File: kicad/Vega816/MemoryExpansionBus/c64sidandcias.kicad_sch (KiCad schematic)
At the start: 7 parts, among them J62 IRQ_OUT, J63 Device Select, J64 A/D Bus, J72 $80 (32B), J76 $00 (16B), J77 $40 (16B)

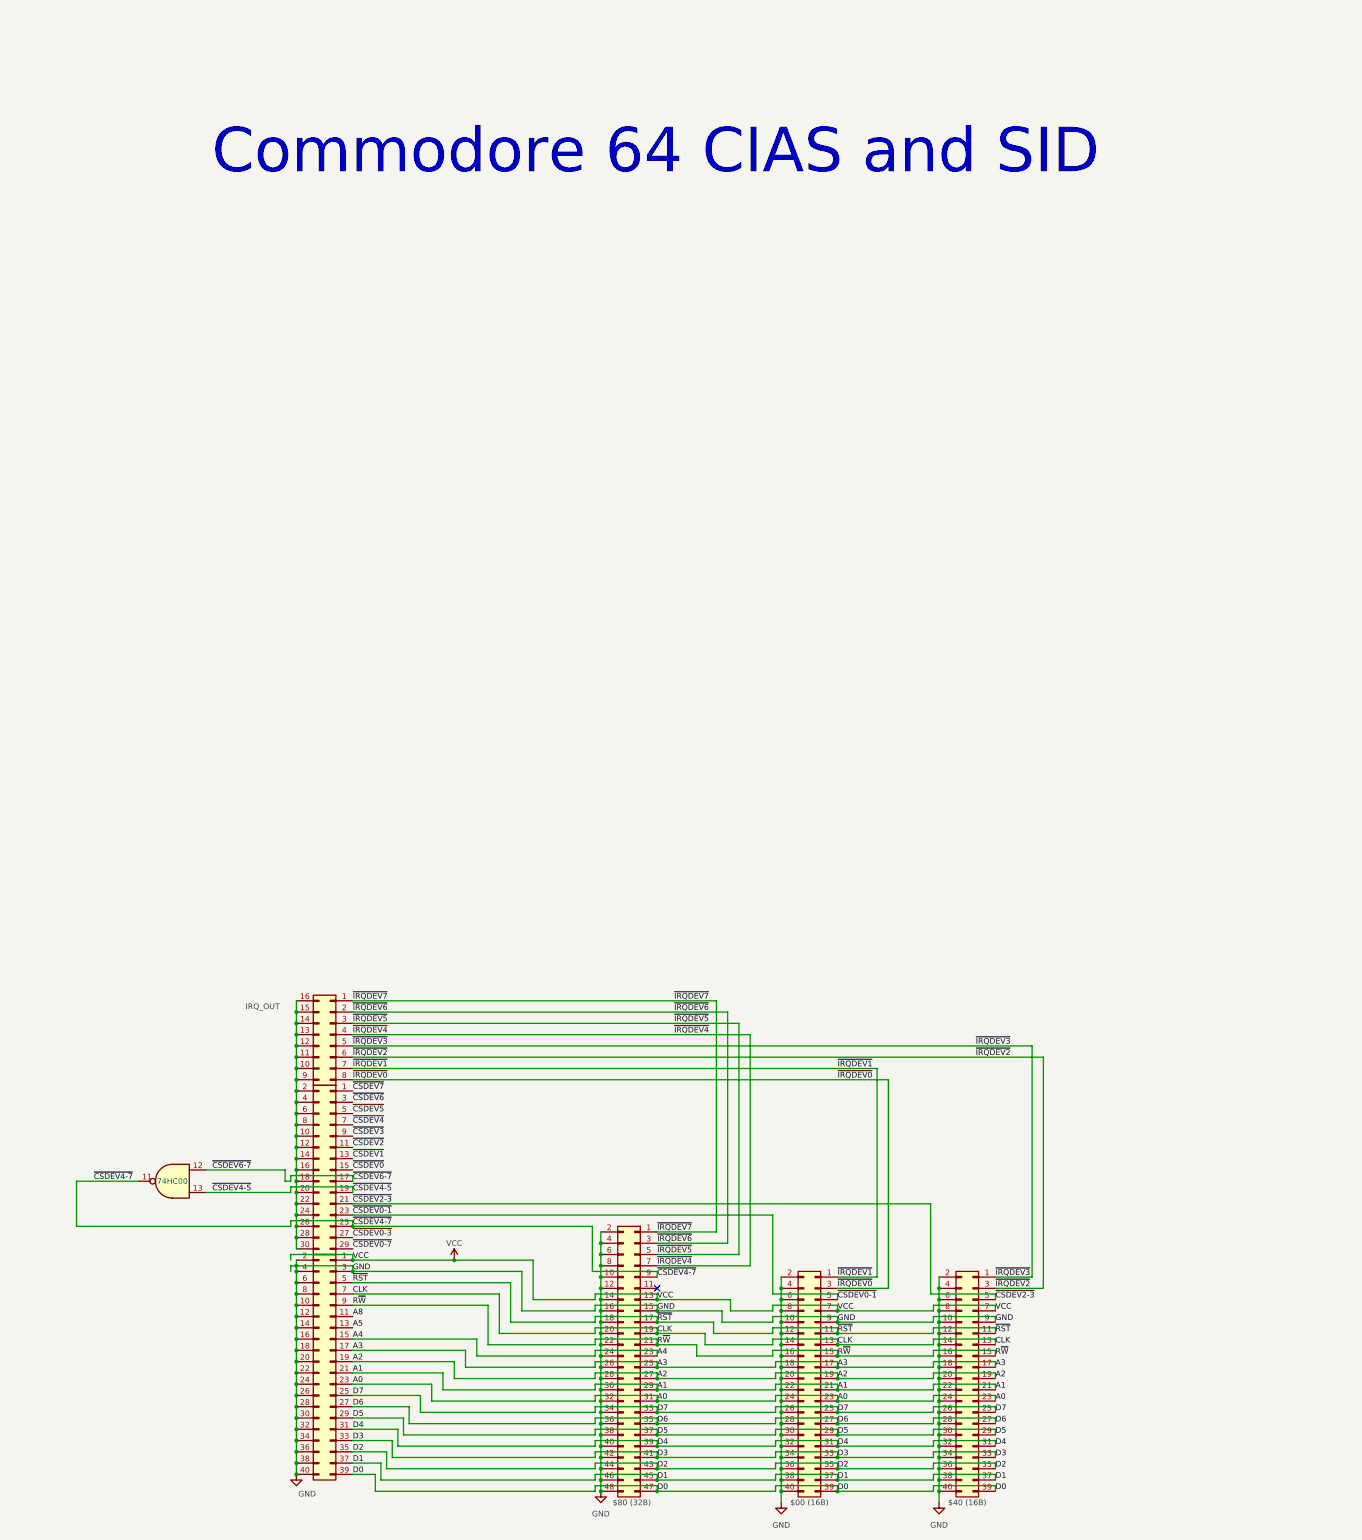
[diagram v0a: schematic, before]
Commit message: expansion port hi ram
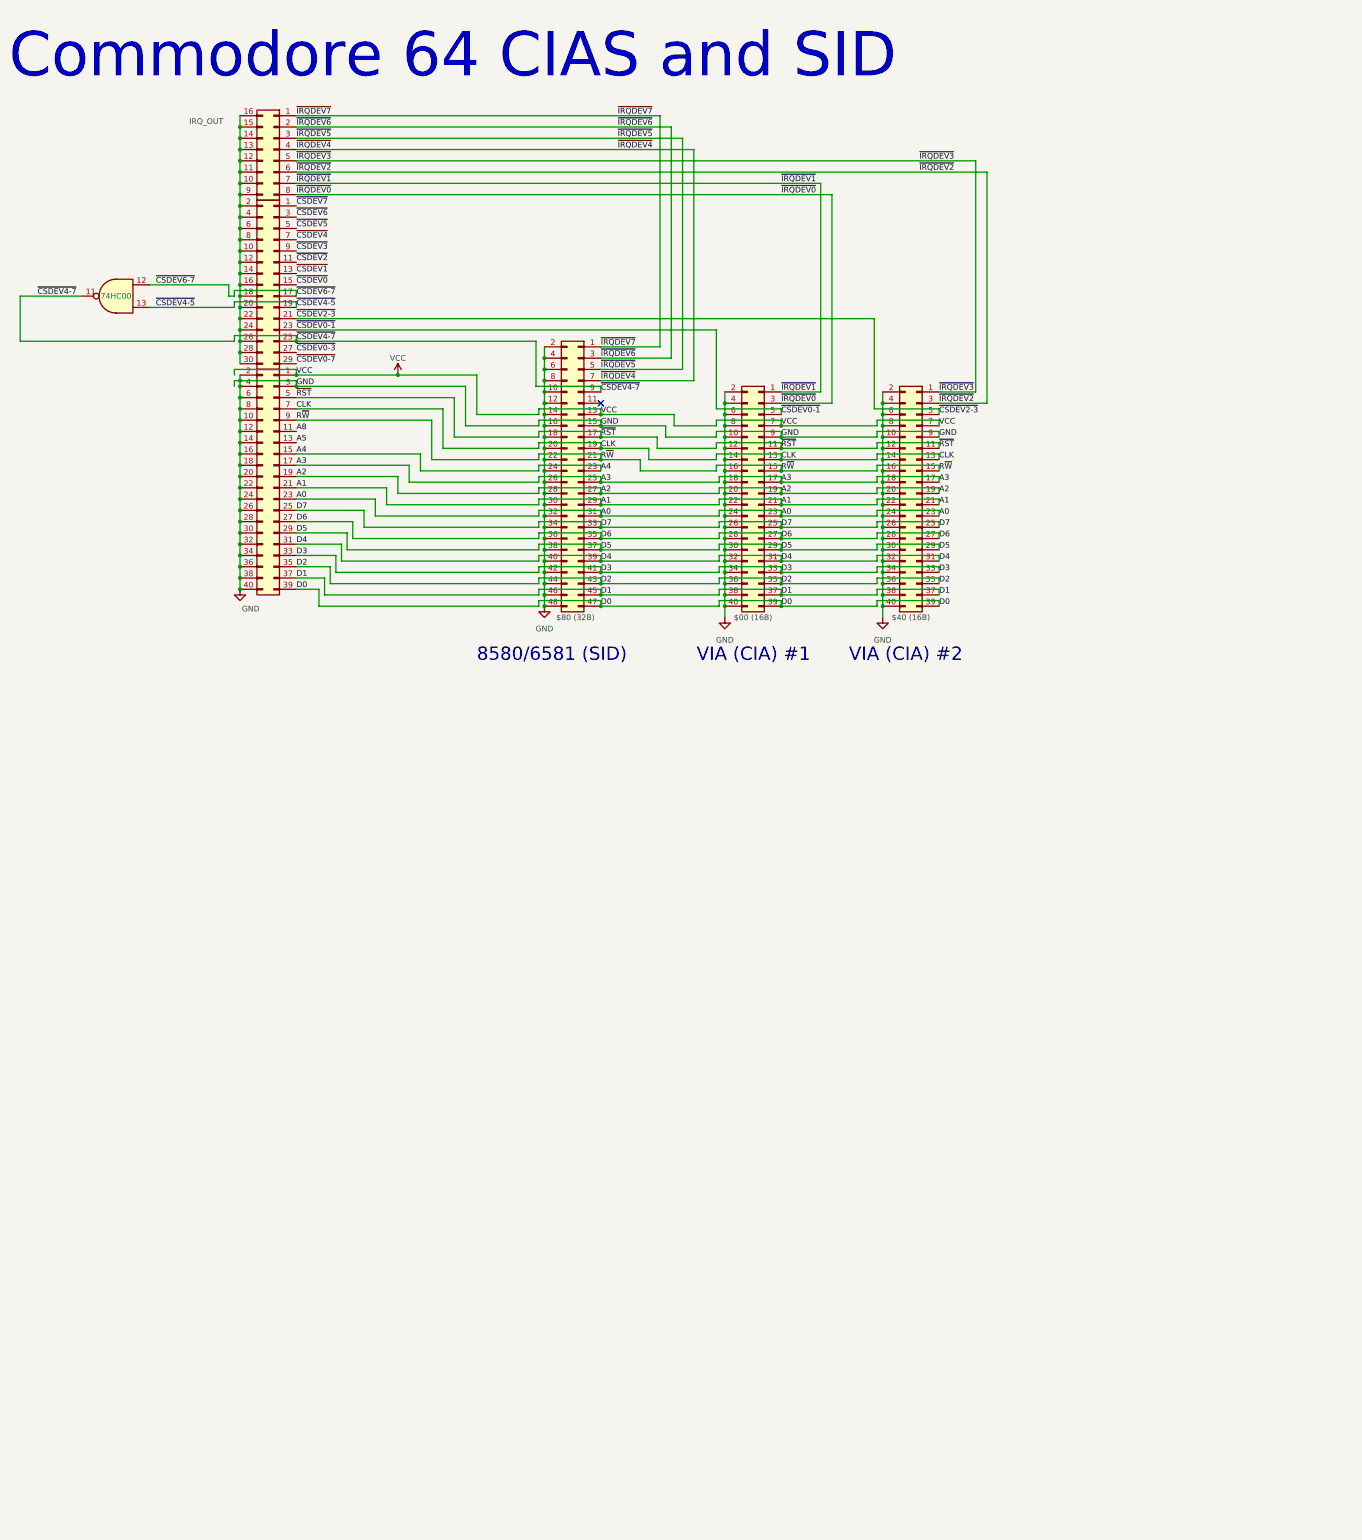
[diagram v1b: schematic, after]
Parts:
- removed U?: 74HC00, symbol 74xx:74HC00
- added U?: 74HC00, symbol 74xx:74HC00
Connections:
- net ~{CSDEV4-5}: now also U?.13
- net ~{CSDEV4-7}: now also U?.11
- net ~{CSDEV6-7}: now also U?.12
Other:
- note added: "8580/6581 (SID)"
- note added: "VIA (CIA) #1"
- note added: "VIA (CIA) #2"
